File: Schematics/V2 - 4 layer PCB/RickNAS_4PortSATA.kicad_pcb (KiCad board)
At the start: 4 copper layers, 32 parts, among them J1 2227595-1, J10 10076579-002C-TRLF, J6 POWER, J7 10076579-002C-TRLF, J8 10076579-002C-TRLF, J9 10076579-002C-TRLF, U1 CH32V003FxPx

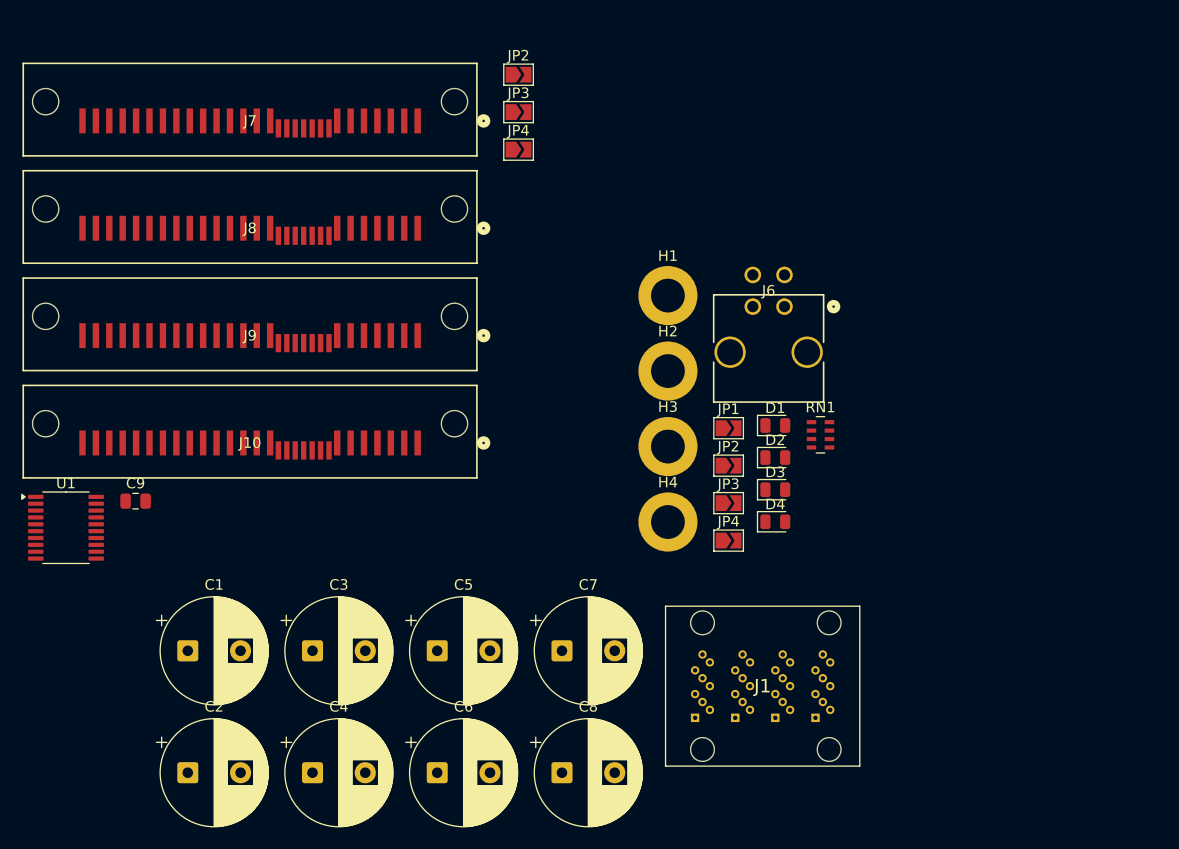
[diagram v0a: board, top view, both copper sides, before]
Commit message: Progress on V2
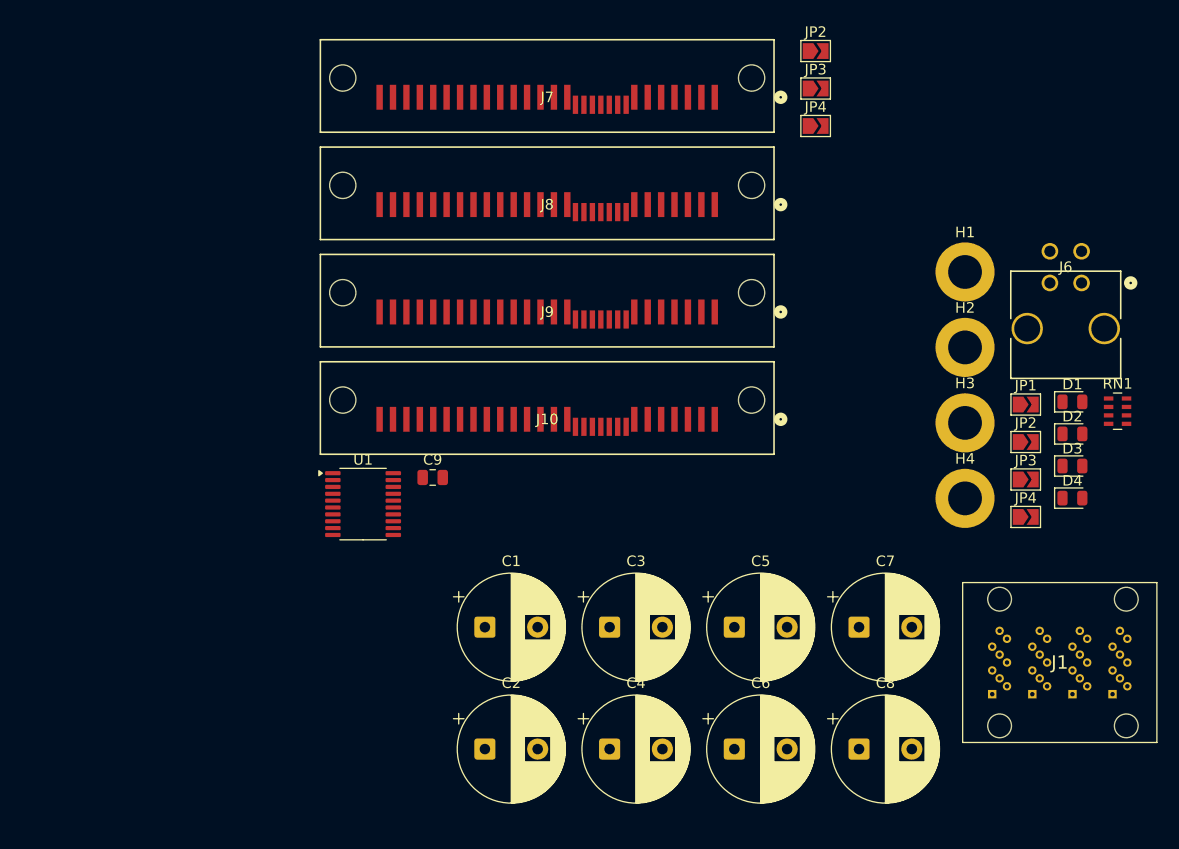
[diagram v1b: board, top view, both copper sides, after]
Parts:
- moved C9 28.2 mm to (128.4, 82.3)
- moved D2 28.2 mm to (189.0, 78.1)
- moved D4 28.2 mm to (189.0, 84.2)
- moved H1 28.2 mm to (178.9, 62.8)
- moved H3 28.2 mm to (178.9, 77.1)
- moved J1 28.2 mm to (192.8, 102.8)
- moved J10 28.2 mm to (139.3, 75.7)
- moved J6 28.2 mm to (189.9, 63.8)
- moved J8 28.2 mm to (139.3, 55.4)
- moved JP2 28.2 mm to (184.6, 78.9)
- moved JP3 28.2 mm to (184.6, 82.5)
- moved JP3 28.2 mm to (164.7, 45.4)
- moved JP4 28.2 mm to (164.7, 49.0)
- moved RN1 28.2 mm to (193.3, 76.0)
- moved C1 28.2 mm to (133.4, 96.5)
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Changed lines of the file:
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@@
 	(footprint "Jumper:SolderJumper-2_P1.3mm_Open_TrianglePad1.0x1.5mm"
 		(layer "F.Cu")
-		(at 136.5584 51.211599)
+		(at 164.704462 48.971599)
 		(descr "SMD Solder Jumper, 1x1.5mm Triangular Pads, 0.3mm gap, open")
 		(tags "solder jumper open")
@@
 	(footprint "LED_SMD:LED_0805_2012Metric"
 		(layer "F.Cu")
-		(at 160.88 77.345)
+		(at 189.026062 75.105)
 		(descr "LED SMD 0805 (2012 Metric), square (rectangular) end terminal, IPC-7351 nominal, (Body size source: https://docs.google.com/spreadsheets/d/1BsfQQcO9C6DZCsRaXUlFlo91Tg2WpOkGARC1WS5S8t0/edit?usp=sharing), generated with kicad-footprint-generator")
 		(tags "LED")
@@
 	(footprint "Capacitor_THT:CP_Radial_D10.0mm_P5.00mm"
 		(layer "F.Cu")
-		(at 140.668584 110.24)
+		(at 168.814646 108)
 		(descr "CP, Radial series, Radial, pin pitch=5.00mm, diameter=10mm, height=16mm, Electrolytic Capacitor")
 		(tags "CP Radial series Radial pin pitch 5.00mm diameter 10mm height 16mm Electrolytic Capacitor")
@@
 	(footprint "Package_SO:TSSOP-20_4.4x6.5mm_P0.65mm"
 		(layer "F.Cu")
-		(at 93.6834 87.031599)
+		(at 121.829462 84.791599)
 		(descr "TSSOP, 20 Pin (JEDEC MO-153 Var AC https://www.jedec.org/document_search?search_api_views_fulltext=MO-153), generated with kicad-footprint-generator ipc_gullwing_generator.py")
 		(tags "TSSOP SO")
@@
 	(footprint "LED_SMD:LED_0805_2012Metric"
 		(layer "F.Cu")
-		(at 160.88 80.385)
+		(at 189.026062 78.145)
 		(descr "LED SMD 0805 (2012 Metric), square (rectangular) end terminal, IPC-7351 nominal, (Body size source: https://docs.google.com/spreadsheets/d/1BsfQQcO9C6DZCsRaXUlFlo91Tg2WpOkGARC1WS5S8t0/edit?usp=sharing), generated with kicad-footprint-generator")
 		(tags "LED")
@@
 	(footprint "Capacitor_THT:CP_Radial_D10.0mm_P5.00mm"
 		(layer "F.Cu")
-		(at 105.224646 110.24)
+		(at 133.370708 108)
 		(descr "CP, Radial series, Radial, pin pitch=5.00mm, diameter=10mm, height=16mm, Electrolytic Capacitor")
 		(tags "CP Radial series Radial pin pitch 5.00mm diameter 10mm height 16mm Electrolytic Capacitor")
@@
 	(footprint "Capacitor_THT:CP_Radial_D10.0mm_P5.00mm"
 		(layer "F.Cu")
-		(at 140.668584 98.69)
+		(at 168.814646 96.45)
 		(descr "CP, Radial series, Radial, pin pitch=5.00mm, diameter=10mm, height=16mm, Electrolytic Capacitor")
 		(tags "CP Radial series Radial pin pitch 5.00mm diameter 10mm height 16mm Electrolytic Capacitor")
@@
 	(footprint "Jumper:SolderJumper-2_P1.3mm_Open_TrianglePad1.0x1.5mm"
 		(layer "F.Cu")
-		(at 156.46 84.7)
+		(at 184.606062 82.46)
 		(descr "SMD Solder Jumper, 1x1.5mm Triangular Pads, 0.3mm gap, open")
 		(tags "solder jumper open")
@@
 	(footprint "MountingHole:MountingHole_3.2mm_M3_DIN965_Pad"
 		(layer "F.Cu")
-		(at 150.71 79.34)
+		(at 178.856062 77.1)
 		(descr "Mounting Hole 3.2mm, M3, generated by kicad-footprint-generator mountinghole.py")
 		(tags "mountinghole M3 DIN965")
@@
 	(footprint "UE_Connector:CONN_SD-43045-008_04_MOL"
 		(layer "F.Cu")
-		(at 161.7511 66.082599)
+		(at 189.897162 63.842599)
 		(tags "430450423 ")
 		(property "Reference" "J6"
@@
 	(footprint "Jumper:SolderJumper-2_P1.3mm_Open_TrianglePad1.0x1.5mm"
 		(layer "F.Cu")
-		(at 136.5584 44.111599)
+		(at 164.704462 41.871599)
 		(descr "SMD Solder Jumper, 1x1.5mm Triangular Pads, 0.3mm gap, open")
 		(tags "solder jumper open")
@@
 	(footprint "MountingHole:MountingHole_3.2mm_M3_DIN965_Pad"
 		(layer "F.Cu")
-		(at 150.71 65.04)
+		(at 178.856062 62.8)
 		(descr "Mounting Hole 3.2mm, M3, generated by kicad-footprint-generator mountinghole.py")
 		(tags "mountinghole M3 DIN965")
@@
 	(footprint "Jumper:SolderJumper-2_P1.3mm_Open_TrianglePad1.0x1.5mm"
 		(layer "F.Cu")
-		(at 156.46 77.6)
+		(at 184.606062 75.36)
 		(descr "SMD Solder Jumper, 1x1.5mm Triangular Pads, 0.3mm gap, open")
 		(tags "solder jumper open")
@@
 	(footprint "MountingHole:MountingHole_3.2mm_M3_DIN965_Pad"
 		(layer "F.Cu")
-		(at 150.71 86.49)
+		(at 178.856062 84.25)
 		(descr "Mounting Hole 3.2mm, M3, generated by kicad-footprint-generator mountinghole.py")
 		(tags "mountinghole M3 DIN965")
@@
 	(footprint "Capacitor_THT:CP_Radial_D10.0mm_P5.00mm"
 		(layer "F.Cu")
-		(at 117.039292 110.24)
+		(at 145.185354 108)
 		(descr "CP, Radial series, Radial, pin pitch=5.00mm, diameter=10mm, height=16mm, Electrolytic Capacitor")
 		(tags "CP Radial series Radial pin pitch 5.00mm diameter 10mm height 16mm Electrolytic Capacitor")
@@
 	(footprint "Capacitor_THT:CP_Radial_D10.0mm_P5.00mm"
 		(layer "F.Cu")
-		(at 128.853938 98.69)
+		(at 157 96.45)
 		(descr "CP, Radial series, Radial, pin pitch=5.00mm, diameter=10mm, height=16mm, Electrolytic Capacitor")
 		(tags "CP Radial series Radial pin pitch 5.00mm diameter 10mm height 16mm Electrolytic Capacitor")
@@
 	(footprint "Jumper:SolderJumper-2_P1.3mm_Open_TrianglePad1.0x1.5mm"
 		(layer "F.Cu")
-		(at 156.46 81.15)
+		(at 184.606062 78.91)
 		(descr "SMD Solder Jumper, 1x1.5mm Triangular Pads, 0.3mm gap, open")
 		(tags "solder jumper open")
@@
 	(footprint "UE_Connector:22275951"
 		(layer "F.Cu")
-		(at 164.685 105.04)
+		(at 192.831062 102.8)
 		(descr "2227595-1-5")
 		(tags "Connector")
@@
 	(footprint "Capacitor_THT:CP_Radial_D10.0mm_P5.00mm"
 		(layer "F.Cu")
-		(at 128.853938 110.24)
+		(at 157 108)
 		(descr "CP, Radial series, Radial, pin pitch=5.00mm, diameter=10mm, height=16mm, Electrolytic Capacitor")
 		(tags "CP Radial series Radial pin pitch 5.00mm diameter 10mm height 16mm Electrolytic Capacitor")
@@
 	(footprint "Jumper:SolderJumper-2_P1.3mm_Open_TrianglePad1.0x1.5mm"
 		(layer "F.Cu")
-		(at 156.46 88.25)
+		(at 184.606062 86.01)
 		(descr "SMD Solder Jumper, 1x1.5mm Triangular Pads, 0.3mm gap, open")
 		(tags "solder jumper open")
@@
 	(footprint "LED_SMD:LED_0805_2012Metric"
 		(layer "F.Cu")
-		(at 160.88 83.425)
+		(at 189.026062 81.185)
 		(descr "LED SMD 0805 (2012 Metric), square (rectangular) end terminal, IPC-7351 nominal, (Body size source: https://docs.google.com/spreadsheets/d/1BsfQQcO9C6DZCsRaXUlFlo91Tg2WpOkGARC1WS5S8t0/edit?usp=sharing), generated with kicad-footprint-generator")
 		(tags "LED")
@@
 	(footprint "Capacitor_THT:CP_Radial_D10.0mm_P5.00mm"
 		(layer "F.Cu")
-		(at 117.039292 98.69)
+		(at 145.185354 96.45)
 		(descr "CP, Radial series, Radial, pin pitch=5.00mm, diameter=10mm, height=16mm, Electrolytic Capacitor")
 		(tags "CP Radial series Radial pin pitch 5.00mm diameter 10mm height 16mm Electrolytic Capacitor")
@@
 	(footprint "UE_Connector:CONN_10076579-002C-TRLF_AMP"
 		(layer "F.Cu")
-		(at 111.125 47.421299)
+		(at 139.271062 45.181299)
 		(tags "10076579-002C-TRLF ")
 		(property "Reference" "J7"
@@
 	(footprint "UE_Connector:CONN_10076579-002C-TRLF_AMP"
 		(layer "F.Cu")
-		(at 111.125 77.929499)
+		(at 139.271062 75.689499)
 		(tags "10076579-002C-TRLF ")
 		(property "Reference" "J10"
@@
 	(footprint "Resistor_SMD:R_Array_Concave_4x0603"
 		(layer "F.Cu")
-		(at 165.16 78.23)
+		(at 193.306062 75.99)
 		(descr "Thick Film Chip Resistor Array, Wave soldering, Vishay CRA06P (see cra06p.pdf)")
 		(tags "resistor array")
@@
 	(footprint "Capacitor_SMD:C_0805_2012Metric"
 		(layer "F.Cu")
-		(at 100.2784 84.511599)
+		(at 128.424462 82.271599)
 		(descr "Capacitor SMD 0805 (2012 Metric), square (rectangular) end terminal, IPC-7351 nominal, (Body size source: IPC-SM-782 page 76, https://www.pcb-3d.com/wordpress/wp-content/uploads/ipc-sm-782a_amendment_1_and_2.pdf, https://docs.google.com/spreadsheets/d/1BsfQQcO9C6DZCsRaXUlFlo91Tg2WpOkGARC1WS5S8t0/edit?usp=sharing), generated with kicad-footprint-generator")
 		(tags "capacitor")
@@
 	(footprint "LED_SMD:LED_0805_2012Metric"
 		(layer "F.Cu")
-		(at 160.88 86.465)
+		(at 189.026062 84.225)
 		(descr "LED SMD 0805 (2012 Metric), square (rectangular) end terminal, IPC-7351 nominal, (Body size source: https://docs.google.com/spreadsheets/d/1BsfQQcO9C6DZCsRaXUlFlo91Tg2WpOkGARC1WS5S8t0/edit?usp=sharing), generated with kicad-footprint-generator")
 		(tags "LED")
@@
 	(footprint "MountingHole:MountingHole_3.2mm_M3_DIN965_Pad"
 		(layer "F.Cu")
-		(at 150.71 72.19)
+		(at 178.856062 69.95)
 		(descr "Mounting Hole 3.2mm, M3, generated by kicad-footprint-generator mountinghole.py")
 		(tags "mountinghole M3 DIN965")
@@
 	(footprint "Jumper:SolderJumper-2_P1.3mm_Open_TrianglePad1.0x1.5mm"
 		(layer "F.Cu")
-		(at 136.5584 47.661599)
+		(at 164.704462 45.421599)
 		(descr "SMD Solder Jumper, 1x1.5mm Triangular Pads, 0.3mm gap, open")
 		(tags "solder jumper open")
@@
 	(footprint "UE_Connector:CONN_10076579-002C-TRLF_AMP"
 		(layer "F.Cu")
-		(at 111.125 67.760099)
+		(at 139.271062 65.520099)
 		(tags "10076579-002C-TRLF ")
 		(property "Reference" "J9"
@@
 	(footprint "UE_Connector:CONN_10076579-002C-TRLF_AMP"
 		(layer "F.Cu")
-		(at 111.125 57.590699)
+		(at 139.271062 55.350699)
 		(tags "10076579-002C-TRLF ")
 		(property "Reference" "J8"
@@
 	(footprint "Capacitor_THT:CP_Radial_D10.0mm_P5.00mm"
 		(layer "F.Cu")
-		(at 105.224646 98.69)
+		(at 133.370708 96.45)
 		(descr "CP, Radial series, Radial, pin pitch=5.00mm, diameter=10mm, height=16mm, Electrolytic Capacitor")
 		(tags "CP Radial series Radial pin pitch 5.00mm diameter 10mm height 16mm Electrolytic Capacitor")
